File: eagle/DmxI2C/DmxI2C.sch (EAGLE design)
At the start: 32 parts, among them IC1 ATMEGA368P-PU, IC2 MAX485, IC5 MC78M12CT, Q1 20MHz

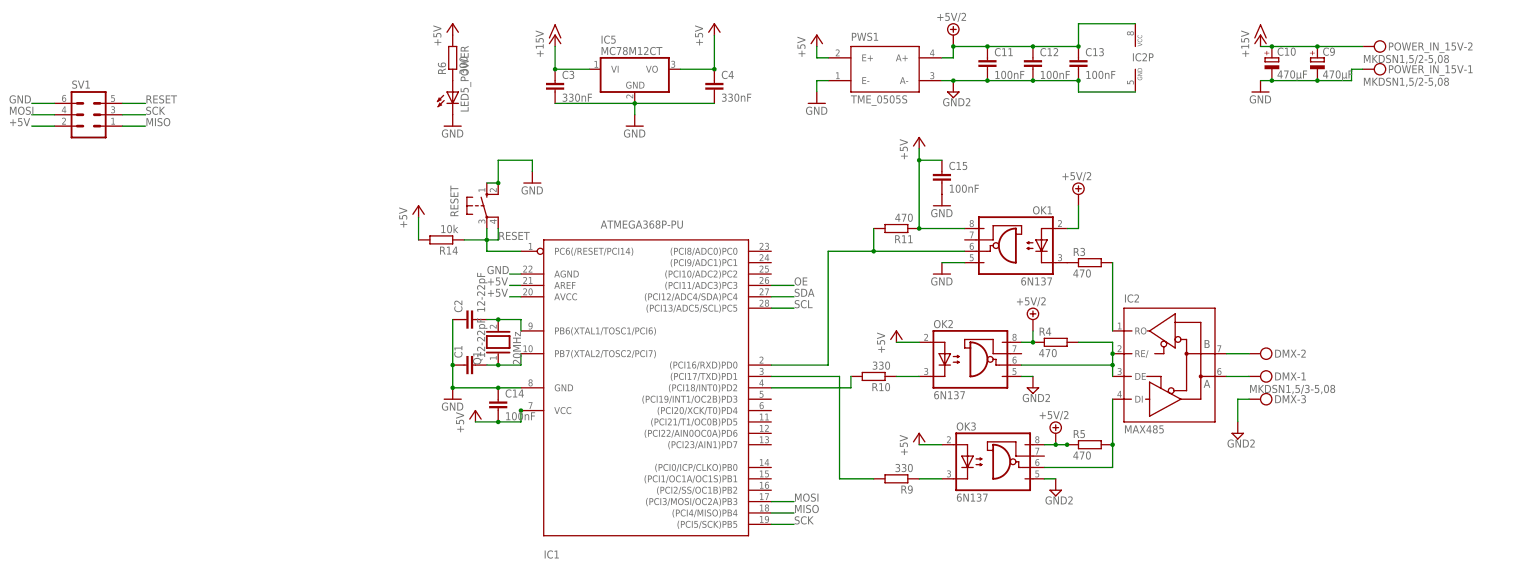
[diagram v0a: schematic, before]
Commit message: routage
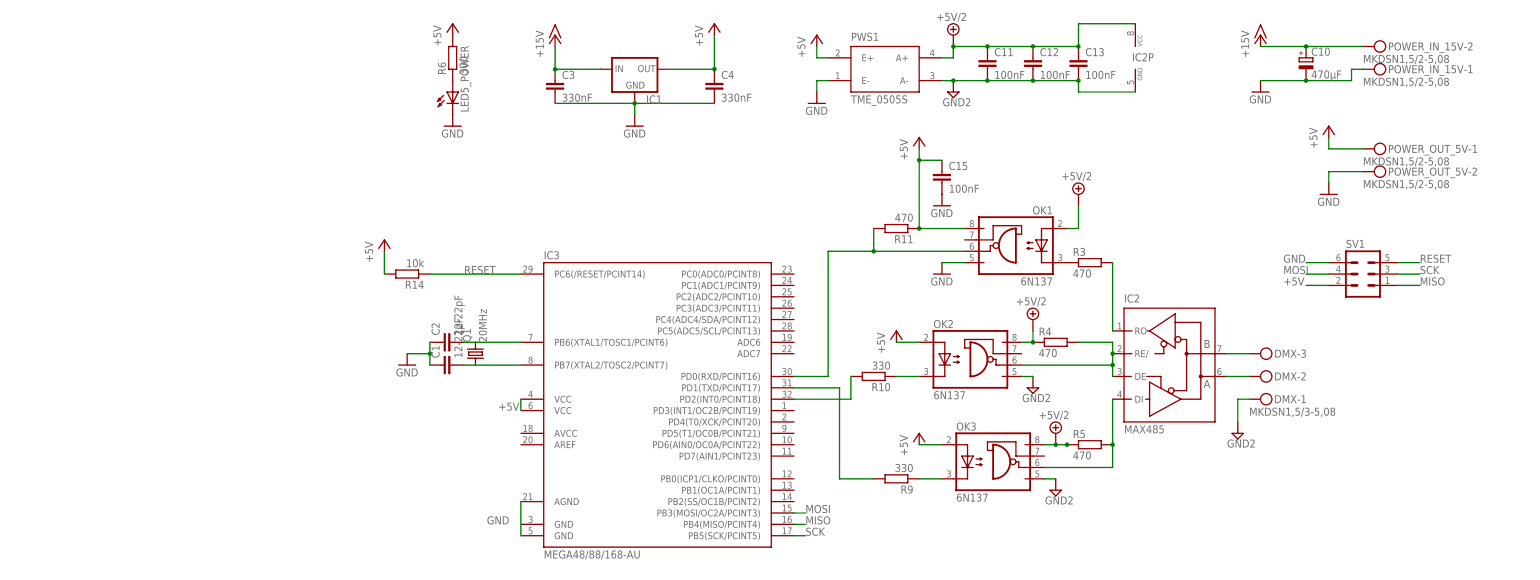
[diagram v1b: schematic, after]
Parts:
- removed C14: 100nF, rcl:C-EU050-025X075
- removed C9: 470µF, rcl:CPOL-EUE5-10.5
- removed IC5: MC78M12CT, linear:MC78M12CT
- removed RESET: (no value), switch-omron:10-XX
- added IC3: MEGA48/88/168-AU, avr-6:MEGA48/88/168-AU
- added POWER_OUT_5V: MKDSN1,5/2-5,08, con-phoenix-508:MKDSN1,5/2-5,08
- C1, C2: device rcl:C-EU025-025X050 -> rcl:C-EUC0805
- C11, C12, C13, C15: device rcl:C-EU050-025X075 -> rcl:C-EUC0805
- IC1: value ATMEGA368P-PU -> (none); device adafruit:ATMEGA168-20P -> v-reg:78XXL
- Q1: device special:XTAL/S -> adafruit:CRYSTALHC49UP
- R10, R11, R3, R4, R5, R9: device rcl:R-EU_0207/7 -> rcl:R-EU_R0805
- R14, R6: device rcl:R-EU_0204/7 -> rcl:R-EU_R0805
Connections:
- removed net N$19: C2.2, IC1.PB6(XTAL1/TOSC1/PCI6), Q1.2
- removed net OE: IC1.(PCI11/ADC3)PC3
- removed net SCL: IC1.(PCI13/ADC5/SCL)PC5
- removed net SDA: IC1.(PCI12/ADC4/SDA)PC4
- new net N$12: IC3.PD1(TXD/PCINT17), R9.2
- net +15V: now also IC1.IN; no longer C9.+, IC5.VI
- net +5V: now also IC1.OUT, IC3.VCC@1, IC3.VCC@2, POWER_OUT_5V-1.KL; no longer C14.2, IC1.AREF, IC1.AVCC, IC1.VCC, IC5.VO
- net GND: now also IC3.AGND, POWER_OUT_5V-2.KL; no longer C14.1, C9.-, IC1.AGND, IC5.GND, RESET.S, RESET.S1
- net GND2: now also DMX-1.KL; no longer DMX-3.KL
- net MISO: now also IC3.PB4(MISO/PCINT4); no longer IC1.(PCI4/MISO)PB4
- net MOSI: now also IC3.PB3(MOSI/OC2A/PCINT3); no longer IC1.(PCI3/MOSI/OC2A)PB3
- net N$10: now also DMX-3.KL; no longer DMX-2.KL
- net N$11: now also DMX-2.KL; no longer DMX-1.KL
- net N$18: now also IC3.PB7(XTAL2/TOSC2/PCINT7); no longer IC1.PB7(XTAL2/TOSC2/PCI7)
- net N$7: now also IC3.PD0(RXD/PCINT16); no longer IC1.(PCI16/RXD)PD0
- net N$8: now also IC3.PD2(INT0/PCINT18); no longer IC1.(PCI18/INT0)PD2
- net N$9: now also C2.2, IC3.PB6(XTAL1/TOSC1/PCINT6), Q1.2; no longer IC1.(PCI17/TXD)PD1, R9.2
- net RESET: now also IC3.PC6(/RESET/PCINT14); no longer IC1.PC6(/RESET/PCI14), RESET.P, RESET.P1
- net SCK: now also IC3.PB5(SCK/PCINT5); no longer IC1.(PCI5/SCK)PB5
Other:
- moved on the sheet: C1, C10, C2, DMX-1, DMX-2, DMX-3, R14, SV1

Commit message: .
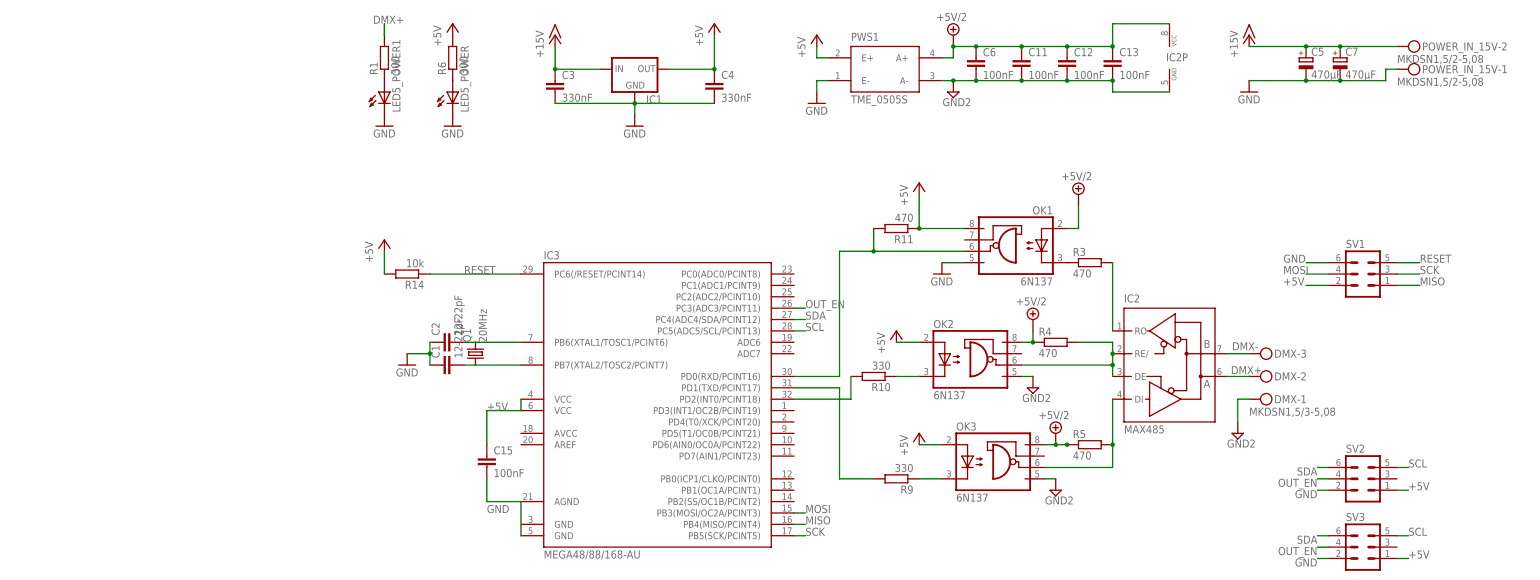
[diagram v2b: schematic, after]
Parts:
- removed C10: 470µF, rcl:CPOL-EUE5-10.5
- removed POWER_OUT_5V: MKDSN1,5/2-5,08, con-phoenix-508:MKDSN1,5/2-5,08
- added C5, C7: 470µF, rcl:CPOL-EUE2.5-6
- added C6: 100nF, rcl:C-EUC0805
- added LED5_POWER1: (no value), led:LED3MM
- added R1: 300, rcl:R-EU_R0805
- added SV2, SV3: (no value), con-lstb:MA03-2
- C3: device rcl:C-EU050-025X075 -> rcl:C-EUC0805
- LED5_POWER: device led:LED5MM -> led:LED3MM
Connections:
- net N$10 renamed DMX-
- removed net N$11: DMX-2.KL, IC2G$1.A
- new net DMX+: DMX-2.KL, IC2G$1.A, R1.2
- new net N$10: LED5_POWER1.A, R1.1
- new net OUT_EN: IC3.PC3(ADC3/PCINT11), SV2.4, SV3.4
- new net SCL: IC3.PC5(ADC5/SCL/PCINT13), SV2.5, SV3.5
- new net SDA: IC3.PC4(ADC4/SDA/PCINT12), SV2.6, SV3.6
- net +15V: now also C5.+, C7.+; no longer C10.+
- net +5V: now also SV2.1, SV3.1; no longer POWER_OUT_5V-1.KL
- net +5V/2: now also C6.1
- net GND: now also C5.-, C7.-, LED5_POWER1.C, SV2.2, SV3.2; no longer C10.-, POWER_OUT_5V-2.KL
- net GND2: now also C6.2
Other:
- moved on the sheet: C11, C12, C13, C15, IC2P, POWER_IN_15V-1, POWER_IN_15V-2
